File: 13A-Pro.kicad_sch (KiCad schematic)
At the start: 30 parts, among them SW1 SW_Push, U1 ProMicro

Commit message: PCB Update
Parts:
- SW1: footprint Button_Switch_SMD:SW_SPST_PTS810 -> Switches:TACTILE_SWITCH_SMD_6.0X3.5MM
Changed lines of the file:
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@@
       (effects (font (size 1.27 1.27)))
     )
-    (property "Footprint" "Button_Switch_SMD:SW_SPST_PTS810" (at 90.17 49.53 0)
+    (property "Footprint" "Switches:TACTILE_SWITCH_SMD_6.0X3.5MM" (at 90.17 49.53 0)
       (effects (font (size 1.27 1.27)) hide)
     )

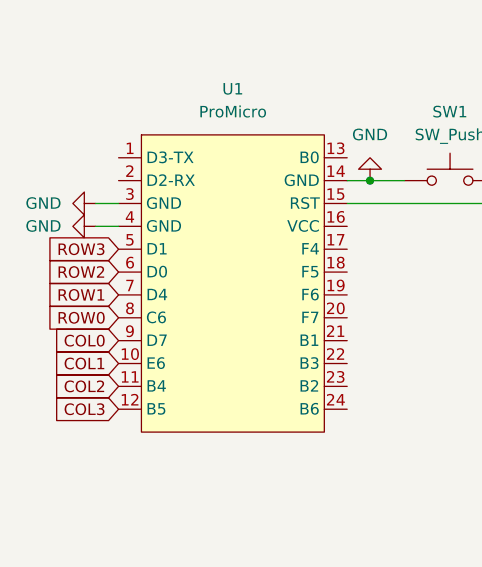
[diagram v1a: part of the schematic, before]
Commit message: PCB Update ver 1.0
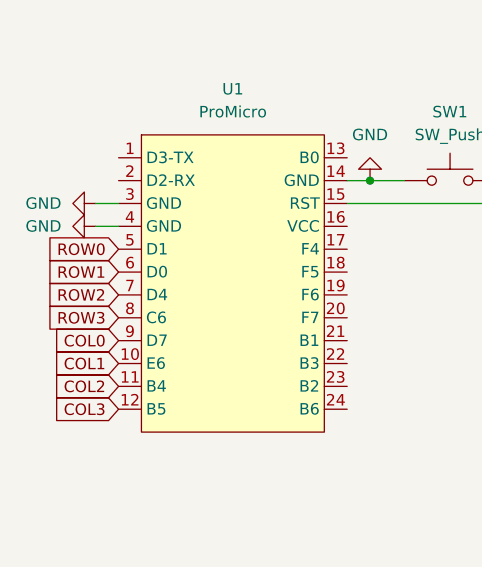
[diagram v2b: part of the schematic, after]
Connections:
- net ROW0: now also U1.5 (D1); no longer U1.8 (C6)
- net ROW1: now also U1.6 (D0); no longer U1.7 (D4)
- net ROW2: now also U1.7 (D4); no longer U1.6 (D0)
- net ROW3: now also U1.8 (C6); no longer U1.5 (D1)
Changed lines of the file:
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@@
     (stroke (width 0) (type default))
   )
-  (global_label "ROW2" (shape input) (at 53.34 64.77 180) (fields_autoplaced)
+  (global_label "ROW2" (shape input) (at 53.34 67.31 180) (fields_autoplaced)
     (effects (font (size 1.27 1.27)) (justify right))
-    (property "Intersheetrefs" "${INTERSHEET_REFS}" (at 45.1728 64.77 0)
+    (property "Intersheetrefs" "${INTERSHEET_REFS}" (at 45.1728 67.31 0)
       (effects (font (size 1.27 1.27)) (justify right) hide)
     )
@@
     )
   )
-  (global_label "ROW0" (shape input) (at 53.34 69.85 180) (fields_autoplaced)
+  (global_label "ROW0" (shape input) (at 53.34 62.23 180) (fields_autoplaced)
     (effects (font (size 1.27 1.27)) (justify right))
-    (property "Intersheetrefs" "${INTERSHEET_REFS}" (at 45.1728 69.85 0)
+    (property "Intersheetrefs" "${INTERSHEET_REFS}" (at 45.1728 62.23 0)
       (effects (font (size 1.27 1.27)) (justify right) hide)
     )
@@
     )
   )
-  (global_label "ROW3" (shape input) (at 53.34 62.23 180) (fields_autoplaced)
+  (global_label "ROW3" (shape input) (at 53.34 69.85 180) (fields_autoplaced)
     (effects (font (size 1.27 1.27)) (justify right))
-    (property "Intersheetrefs" "${INTERSHEET_REFS}" (at 45.1728 62.23 0)
+    (property "Intersheetrefs" "${INTERSHEET_REFS}" (at 45.1728 69.85 0)
       (effects (font (size 1.27 1.27)) (justify right) hide)
     )
   )
-  (global_label "ROW1" (shape input) (at 53.34 67.31 180) (fields_autoplaced)
+  (global_label "ROW1" (shape input) (at 53.34 64.77 180) (fields_autoplaced)
     (effects (font (size 1.27 1.27)) (justify right))
-    (property "Intersheetrefs" "${INTERSHEET_REFS}" (at 45.1728 67.31 0)
+    (property "Intersheetrefs" "${INTERSHEET_REFS}" (at 45.1728 64.77 0)
       (effects (font (size 1.27 1.27)) (justify right) hide)
     )

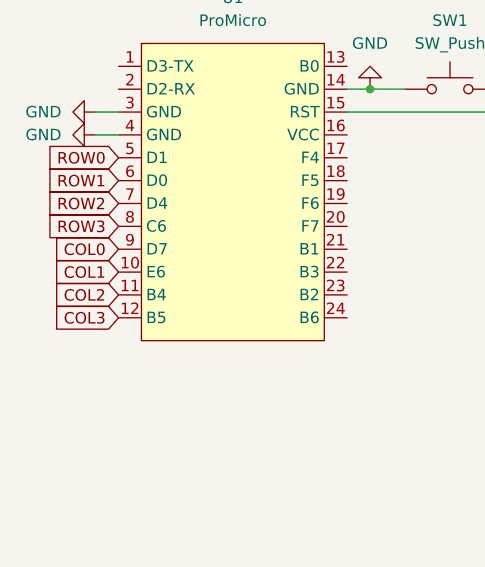
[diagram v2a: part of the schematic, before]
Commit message: Case, PCB, Firmware update
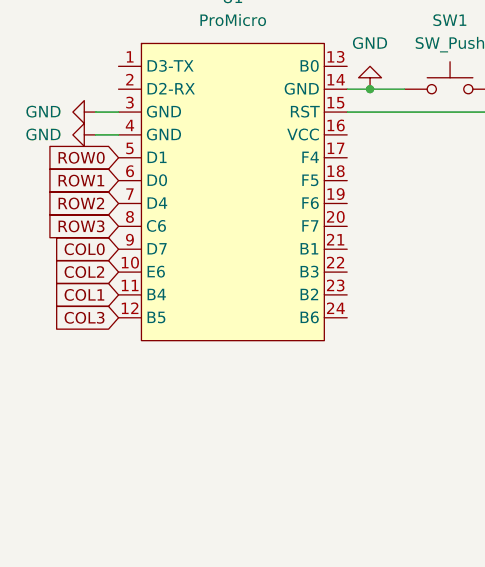
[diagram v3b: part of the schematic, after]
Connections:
- net COL1: now also U1.11 (B4); no longer U1.10 (E6)
- net COL2: now also U1.10 (E6); no longer U1.11 (B4)
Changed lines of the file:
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@@
     )
   )
-  (global_label "COL1" (shape input) (at 53.34 74.93 180) (fields_autoplaced)
+  (global_label "COL1" (shape input) (at 53.34 77.47 180) (fields_autoplaced)
     (effects (font (size 1.27 1.27)) (justify right))
-    (property "Intersheetrefs" "${INTERSHEET_REFS}" (at 45.5961 74.93 0)
+    (property "Intersheetrefs" "${INTERSHEET_REFS}" (at 45.5961 77.47 0)
       (effects (font (size 1.27 1.27)) (justify right) hide)
     )
@@
     )
   )
-  (global_label "COL2" (shape input) (at 53.34 77.47 180) (fields_autoplaced)
+  (global_label "COL2" (shape input) (at 53.34 74.93 180) (fields_autoplaced)
     (effects (font (size 1.27 1.27)) (justify right))
-    (property "Intersheetrefs" "${INTERSHEET_REFS}" (at 45.5961 77.47 0)
+    (property "Intersheetrefs" "${INTERSHEET_REFS}" (at 45.5961 74.93 0)
       (effects (font (size 1.27 1.27)) (justify right) hide)
     )
